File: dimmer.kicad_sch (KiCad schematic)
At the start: 53 parts, among them J1 Screw_Terminal_01x07, J2 Screw_Terminal_01x02, J3 KNX-IN, J4 Screw_Terminal_01x08, Q1 2N2222A, Q10 2N2222A, Q11 2N2222A, Q12 IRFZ44N, Q13 2N2222A, Q14 2N2222A, Q15 IRFZ44N, Q16 2N2222A, Q17 2N2222A, Q18 IRFZ44N, Q2 2N2222A, Q3 IRFZ44N, Q4 2N2222A, Q5 2N2222A, Q6 IRFZ44N, Q7 2N2222A, Q8 2N2222A, Q9 IRFZ44N, U1 L7805, U2 ESP32-DEVKITC-32D

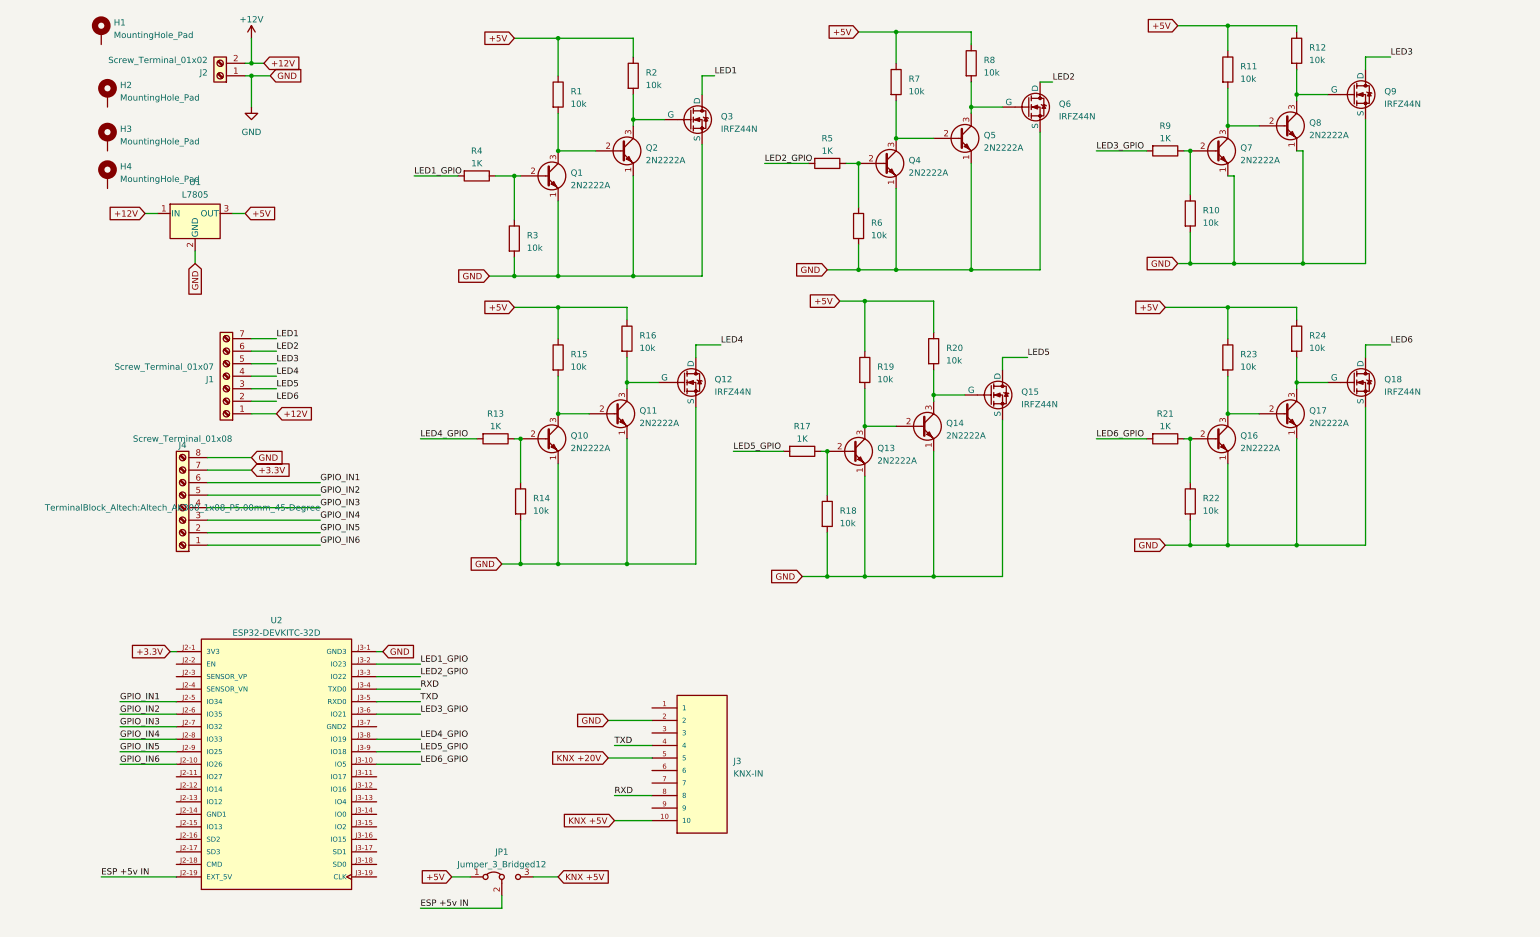
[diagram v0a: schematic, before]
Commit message: Cleanup Schematics
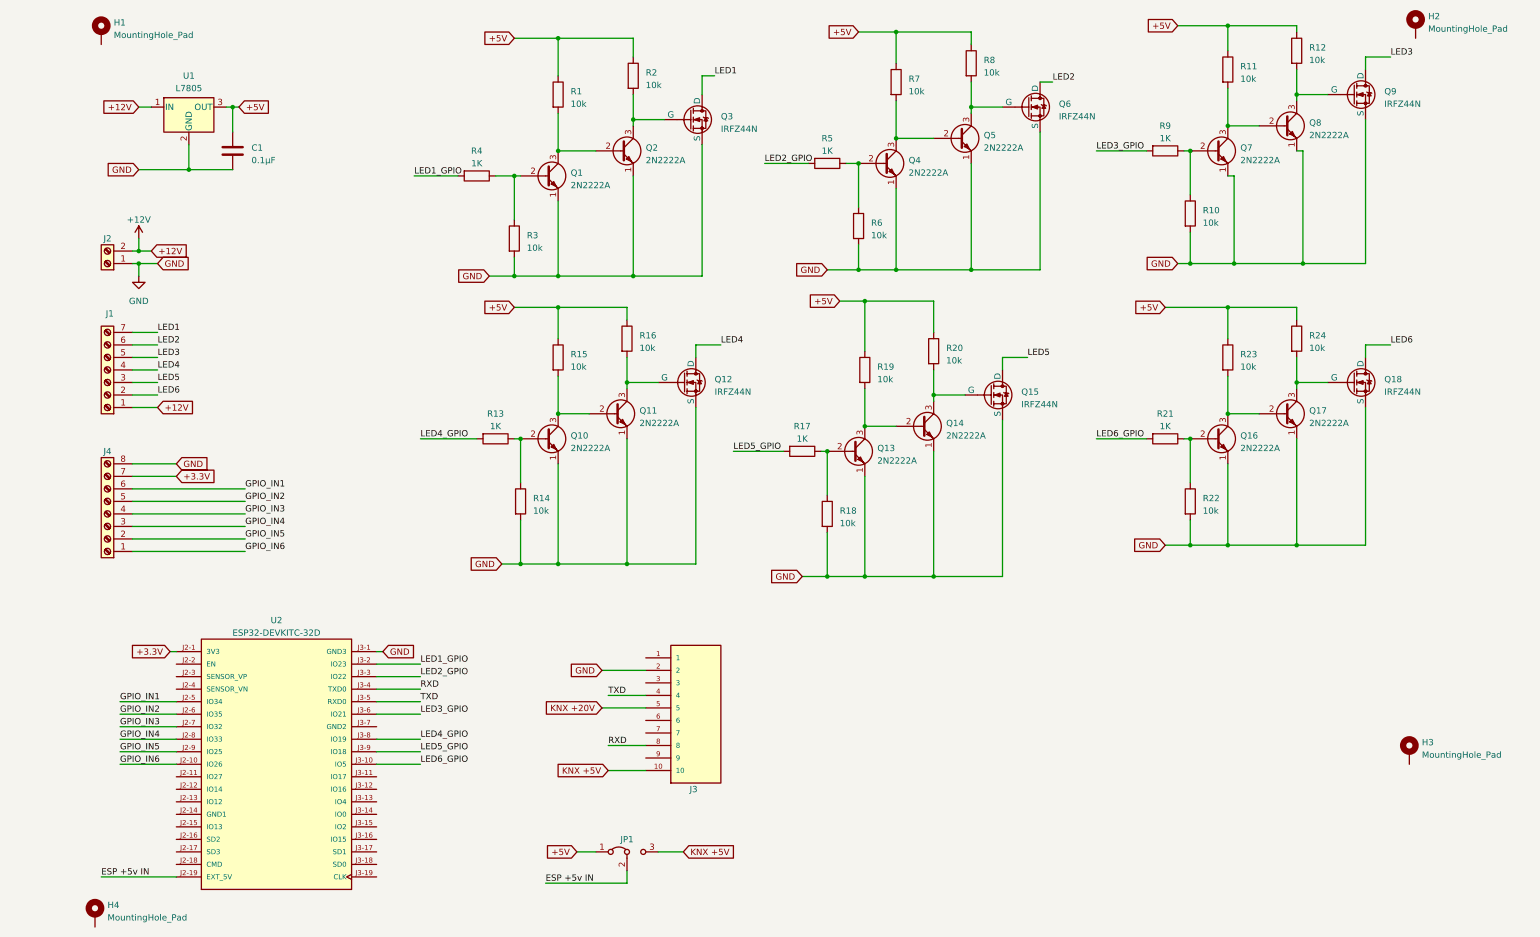
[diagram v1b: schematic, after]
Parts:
- added C1: 0.1μF, Capacitor_THT:CP_Radial_D4.0mm_P1.50mm, symbol Device:C
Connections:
- net +5V: now also C1.1
- net GND: now also C1.2
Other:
- moved on the sheet: H2, H3, H4, J1, J2, J3, J4, JP1, U1
